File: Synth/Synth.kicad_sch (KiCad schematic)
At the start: 0 parts

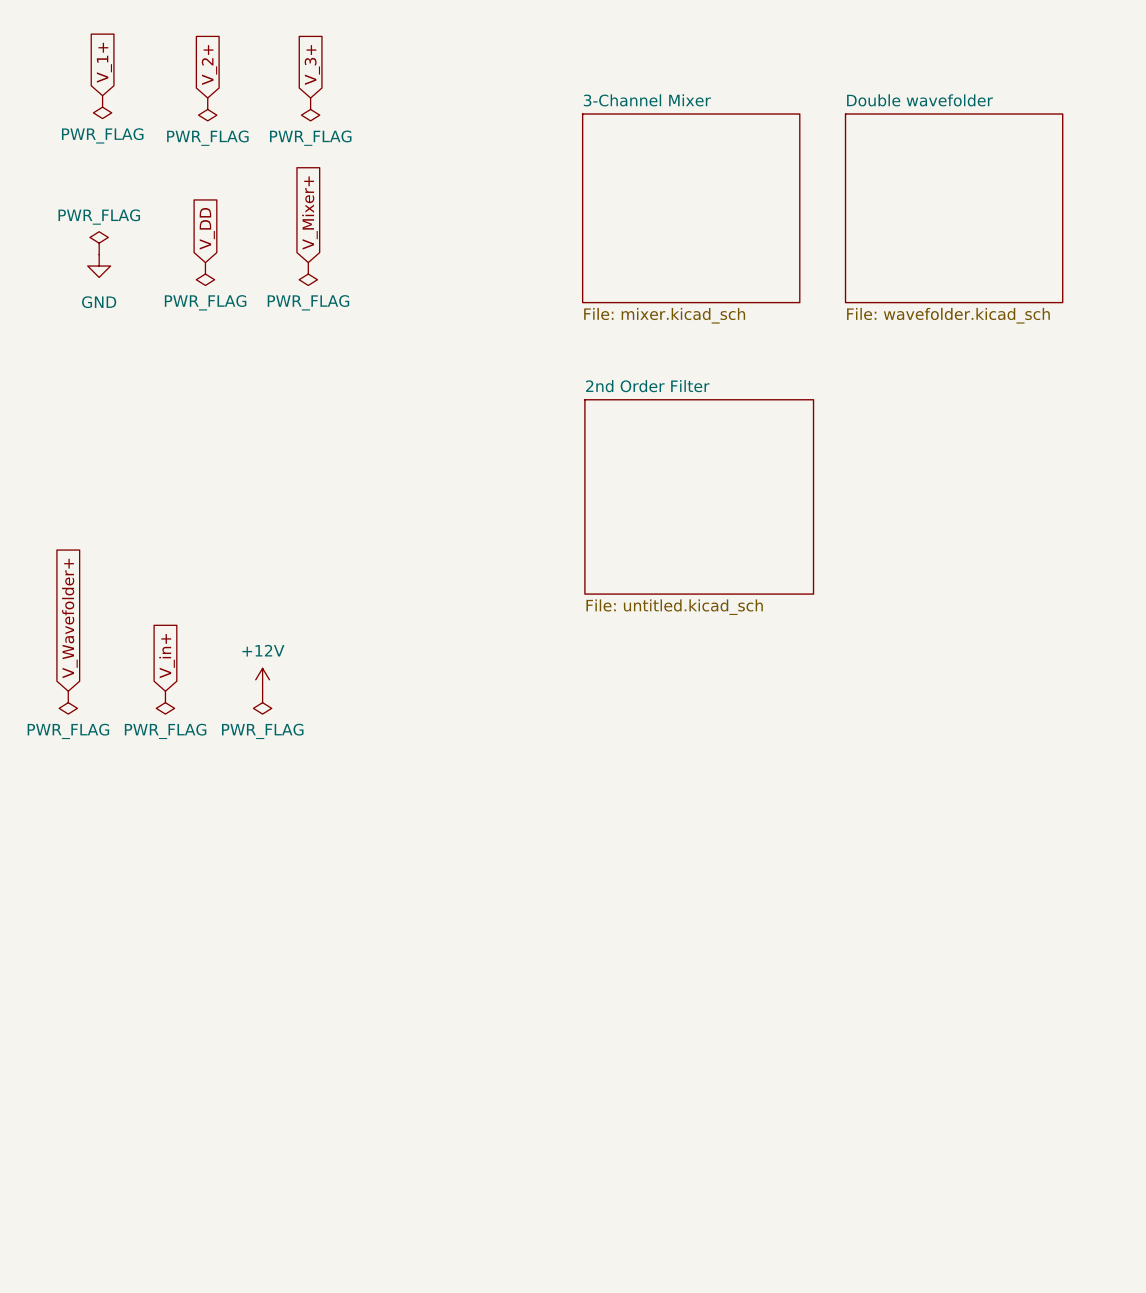
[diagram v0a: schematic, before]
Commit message: fixed erge stuff fingers crossed
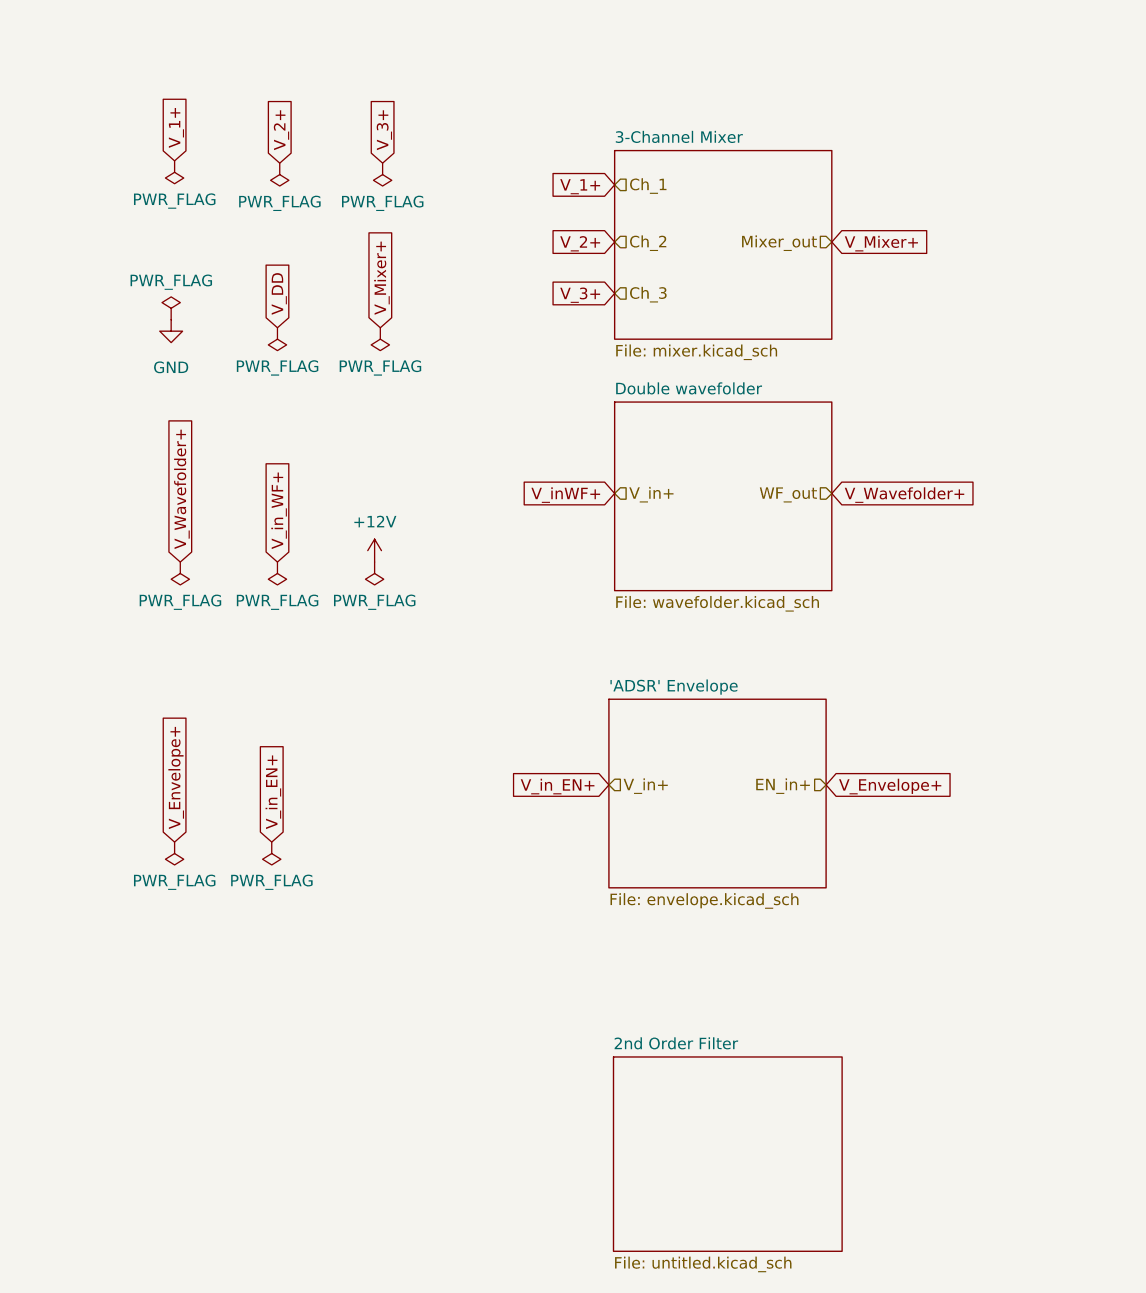
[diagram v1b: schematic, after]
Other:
- added sheet 'ADSR' Envelope (envelope.kicad_sch)
